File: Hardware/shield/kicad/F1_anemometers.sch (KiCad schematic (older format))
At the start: 22 parts, among them U1 MCP6244

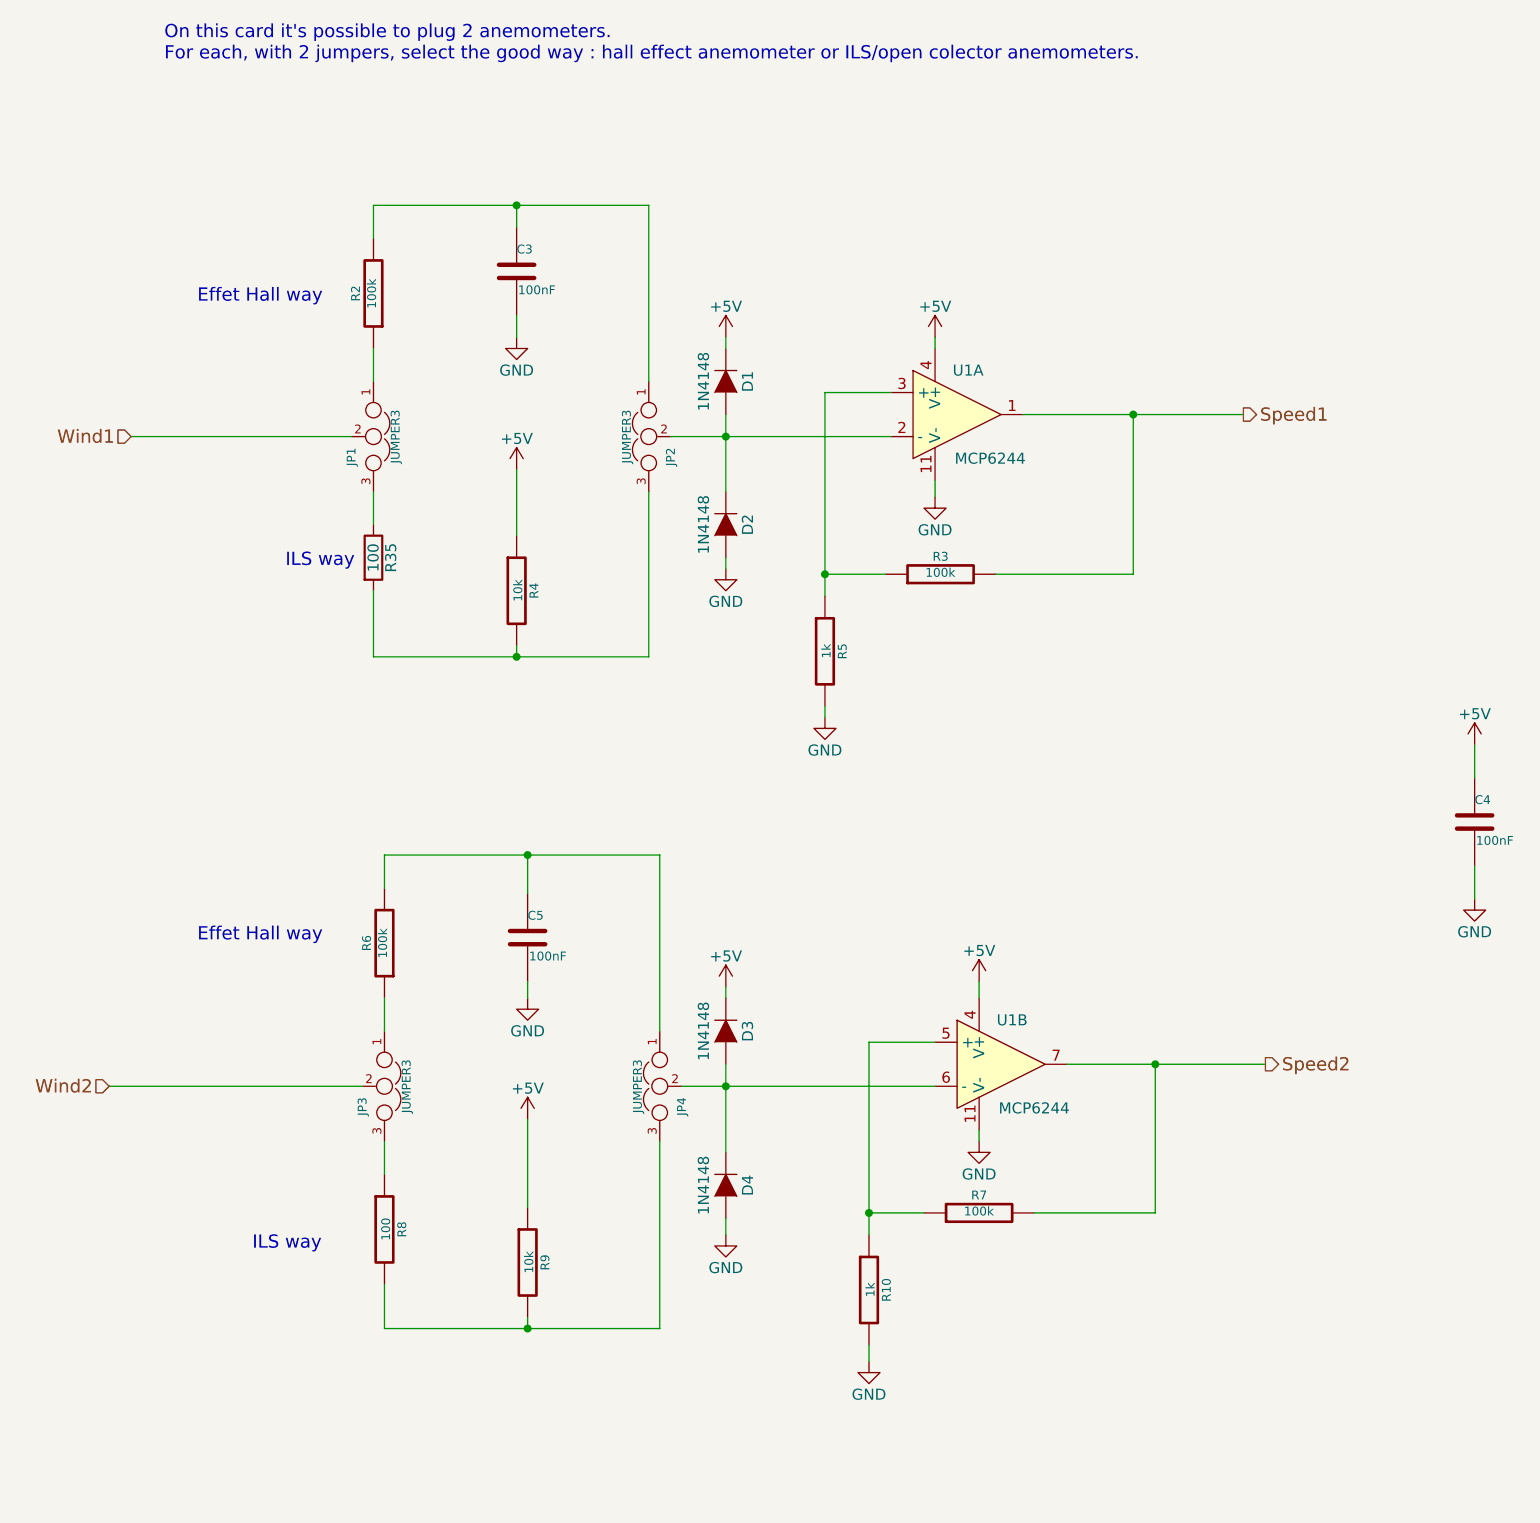
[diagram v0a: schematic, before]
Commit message: move to digital 1.1.1
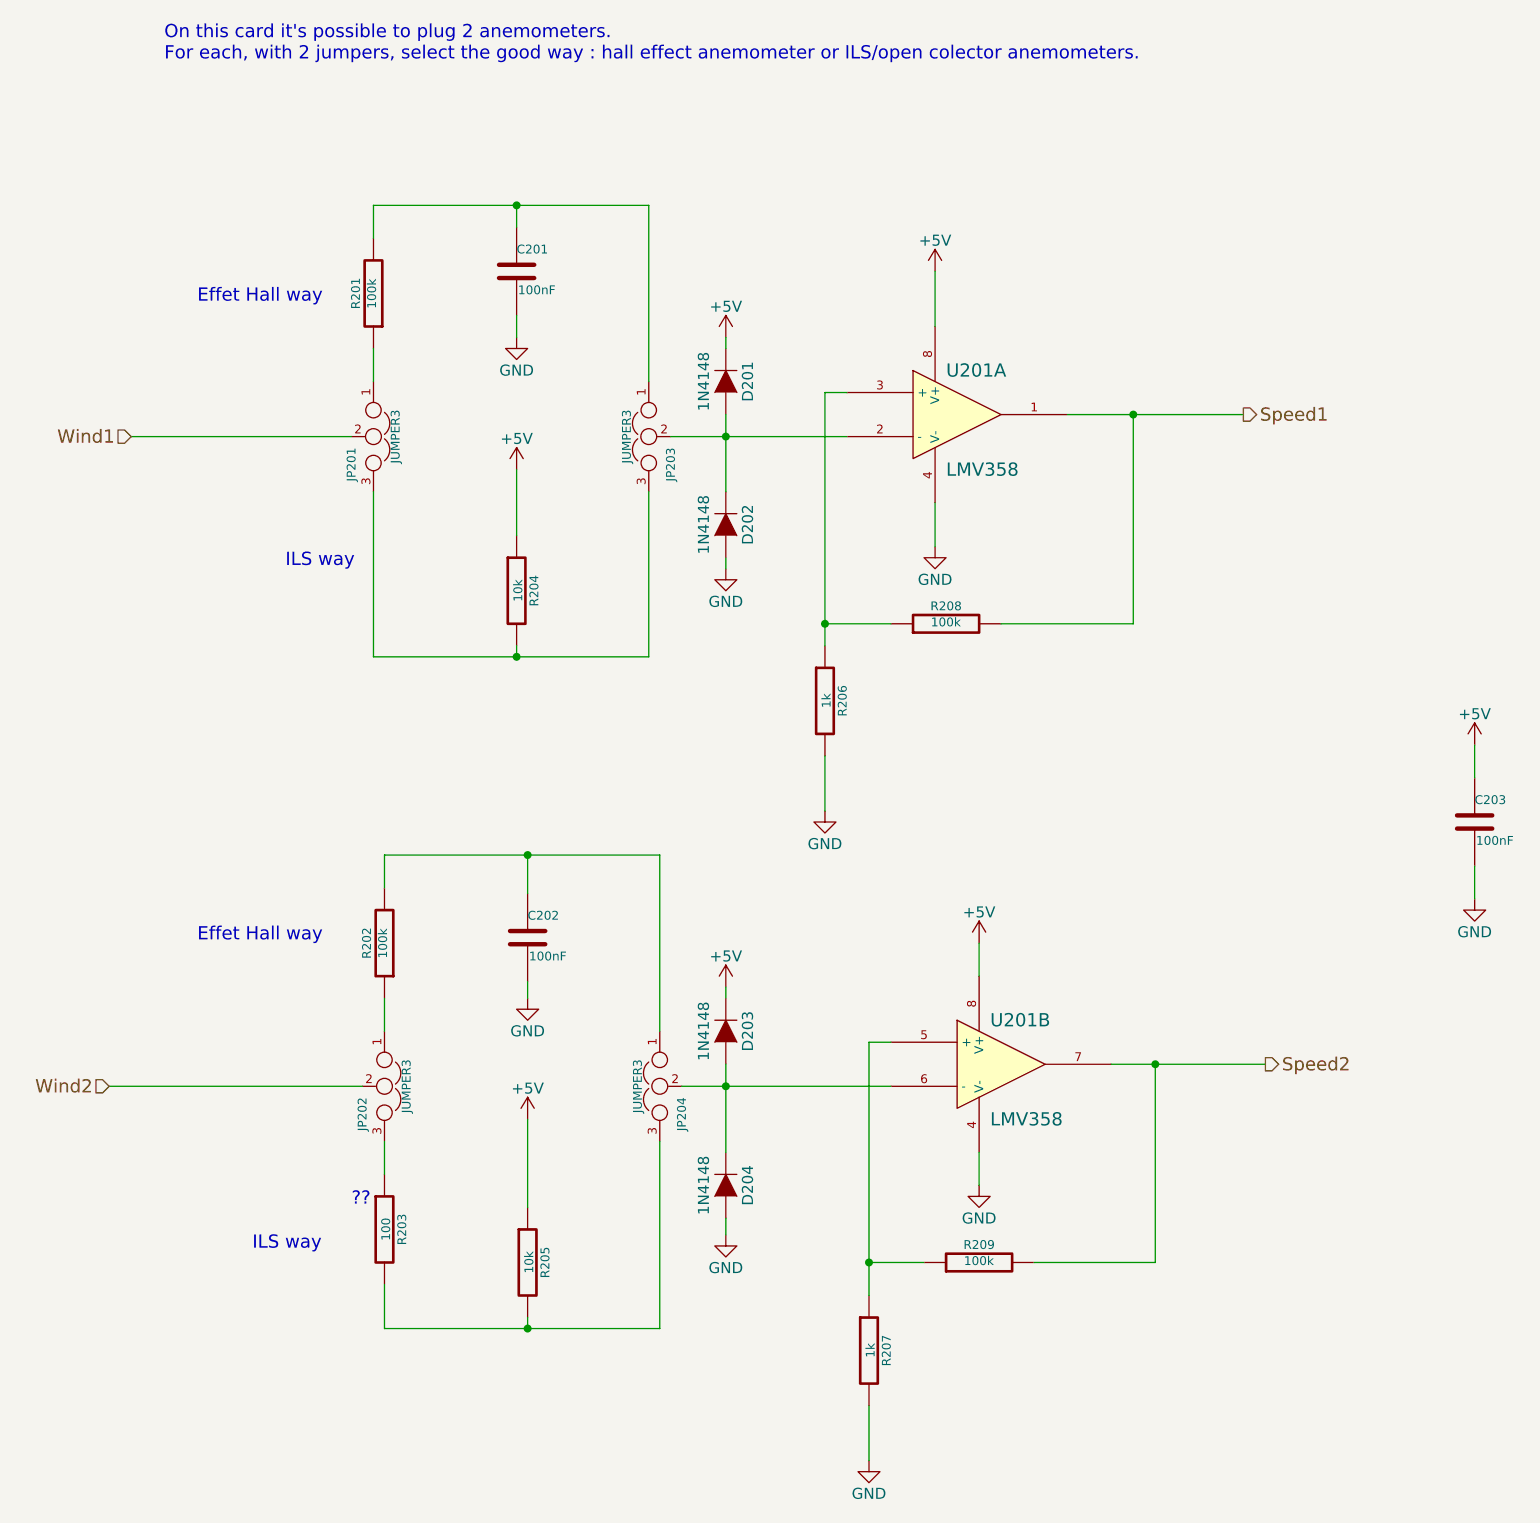
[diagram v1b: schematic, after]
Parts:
- removed R35: 100, Discret:R3-LARGE_PADS, symbol R
- removed U1: MCP6244, Housings_DIP:DIP-14_W7.62mm_LongPads, symbol MCP6004
- added U201: LMV358, Housings_DIP:DIP-8_W7.62mm_LongPads, symbol LM358-RESCUE-Windlogger
- D201: renamed from D1; footprint Discret:DO-35 -> Diodes_ThroughHole:Diode_DO-35_SOD27_Horizontal_RM10
- D202: renamed from D2; footprint Discret:DO-35 -> Diodes_ThroughHole:Diode_DO-35_SOD27_Horizontal_RM10
- D203: renamed from D3; footprint Discret:DO-35 -> Diodes_ThroughHole:Diode_DO-35_SOD27_Horizontal_RM10
- D204: renamed from D4; footprint Discret:DO-35 -> Diodes_ThroughHole:Diode_DO-35_SOD27_Horizontal_RM10
- R201: renamed from R2; footprint Discret:R3-LARGE_PADS -> Discret:R4
- R202: renamed from R6; footprint Discret:R3-LARGE_PADS -> Discret:R4
- R203: renamed from R8; footprint Discret:R3-LARGE_PADS -> Discret:R4
- R204: renamed from R4; footprint Discret:R3-LARGE_PADS -> Discret:R4
- R205: renamed from R9; footprint Discret:R3-LARGE_PADS -> Discret:R4
- R206: renamed from R5; footprint Discret:R3-LARGE_PADS -> Discret:R4
- R207: renamed from R10; footprint Discret:R3-LARGE_PADS -> Discret:R4
- R208: renamed from R3; footprint Discret:R3-LARGE_PADS -> Discret:R4
- R209: renamed from R7; footprint Discret:R3-LARGE_PADS -> Discret:R4
- renumbered C3 to C201, C5 to C202, C4 to C203, JP1 to JP201, JP3 to JP202, JP2 to JP203, JP4 to JP204
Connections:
- net +5V: now also U201.8 (V+), U201.8 (V+)
- net GND: now also U201.4 (V-), U201.4 (V-)
- net Speed1: now also U201.1
- net Speed2: now also U201.7
- net at R206.1, R208.1: now also U201.3 (+)
- net at R207.1, R209.1: now also U201.5 (+)
- net at JP201.3: now also JP203.3, R204.2
- net at D201.2 (A), D202.1 (K), JP203.2: now also U201.2 (-)
- net at D203.2 (A), D204.1 (K), JP204.2: now also U201.6 (-)
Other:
- note added: "??"
- moved on the sheet: R206, R207, R208, R209
